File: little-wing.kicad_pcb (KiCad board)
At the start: 4 copper layers, 119.8 x 94.8 mm, 72 parts, among them IC1 AP7335-WG-7, J1 nice!view, J2 Battery, J3 trackball, J4 trackball, SW1 Power, SW2 Reset, U1 nice!nano v2, U2 PMW3610

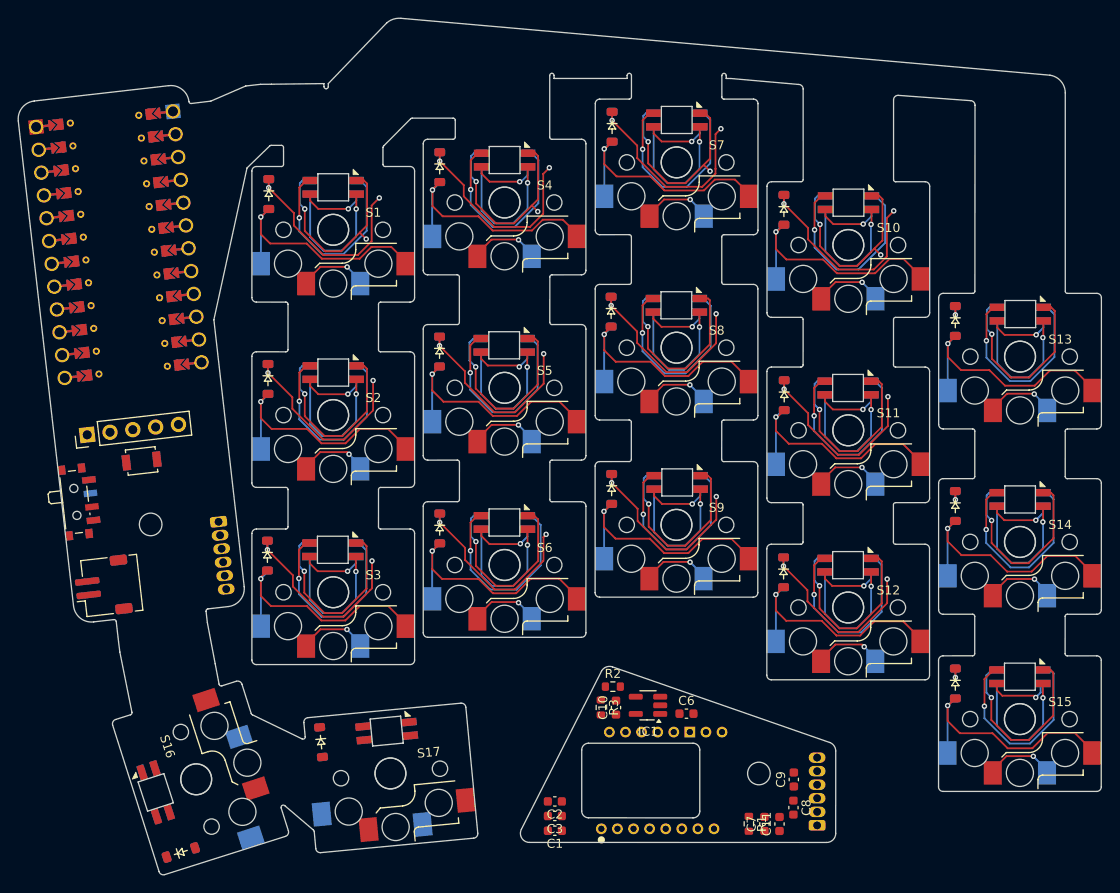
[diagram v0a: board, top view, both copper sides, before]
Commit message: Cleaning up the columns wiring
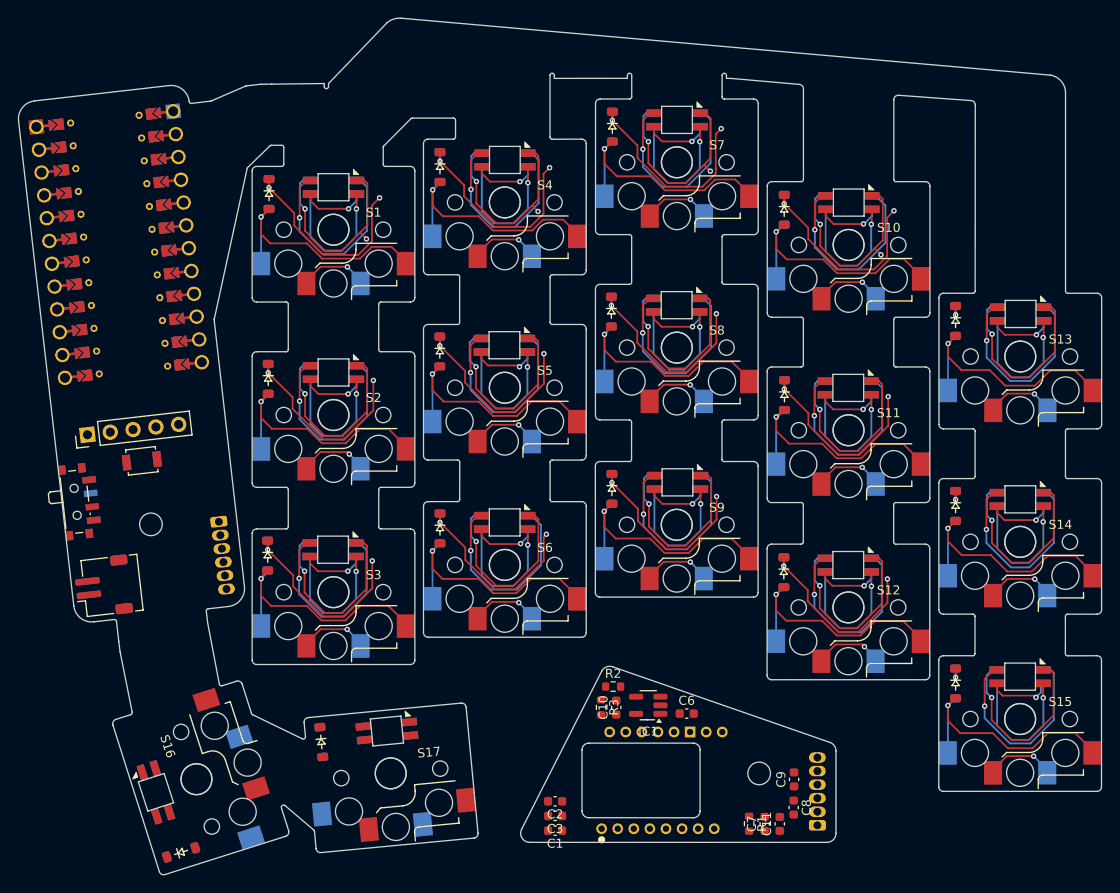
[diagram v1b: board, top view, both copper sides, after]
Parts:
- turned S14 to -1.77636e-15 degrees
- turned S10 to -1.77636e-15 degrees
- turned D31 to -1.77636e-15 degrees
- turned D27 to -1.77636e-15 degrees
- turned D29 to -1.77636e-15 degrees
- turned D33 to -1.77636e-15 degrees
- turned S3 to -1.77636e-15 degrees
- turned S1 to -1.77636e-15 degrees
- turned S7 to -1.77636e-15 degrees
- turned D21 to -1.77636e-15 degrees
- turned D23 to -1.77636e-15 degrees
- turned S4 to -1.77636e-15 degrees
- turned S6 to -1.77636e-15 degrees
- turned D30 to -1.77636e-15 degrees
- turned D26 to -1.77636e-15 degrees
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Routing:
- net VCC: track 556.5 -> 550.0 mm
- net GND: track 706.8 -> 712.6 mm
- net Net-(D19-DIN): track 32.4 -> 37.5 mm
- net Col 0: track 190.9 -> 195.1 mm
- net Row 2: track 244.0 -> 247.5 mm
- net Row 1: track 447.6 -> 450.9 mm
- net Row 0: track 646.0 -> 648.8 mm
- net Col 3: track 122.0 -> 124.5 mm
- net Col 2: track 136.4 -> 138.7 mm
- net Col 1: track 164.1 -> 165.9 mm
- net RGB: track 175.1 -> 176.4 mm
- net Col 4: track 94.5 -> 95.6 mm
- net Net-(D22-DIN): track 106.6 -> 107.7 mm
